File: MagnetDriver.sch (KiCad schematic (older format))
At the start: 54 parts, among them J1 MAGNET1, J2 MAGNET2, J3 INPUT_JACK, J4 PWR_IN, Q1 2N3904, Q2 TIP122, Q3 TIP32A, Q4 2N3904, Q5 TIP122, Q6 TIP32A, U1 LM324, U2 TEENSY_3.6_MINIMAL, U3 LM7805_TO220

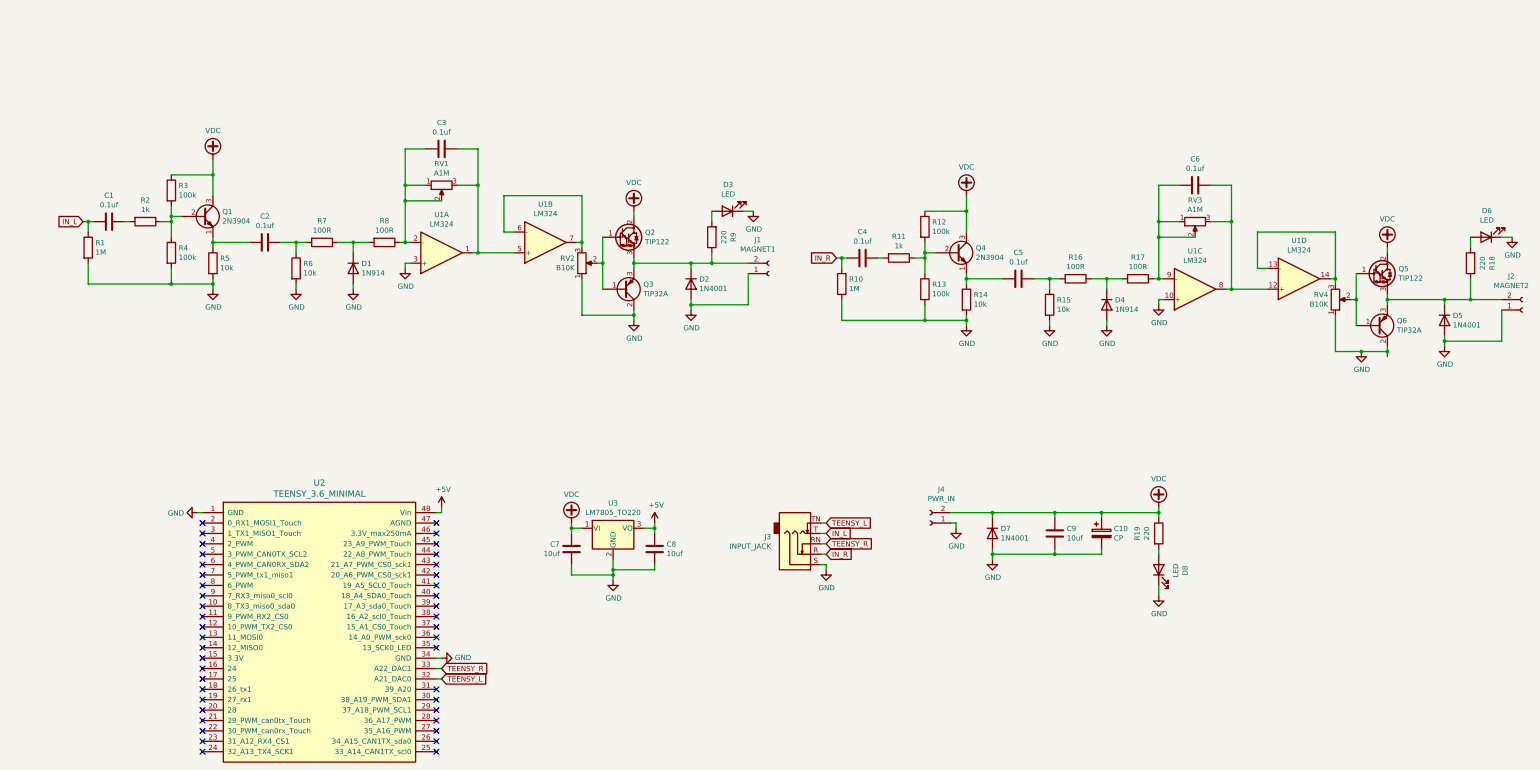
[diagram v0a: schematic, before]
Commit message: checked schematic + footprints
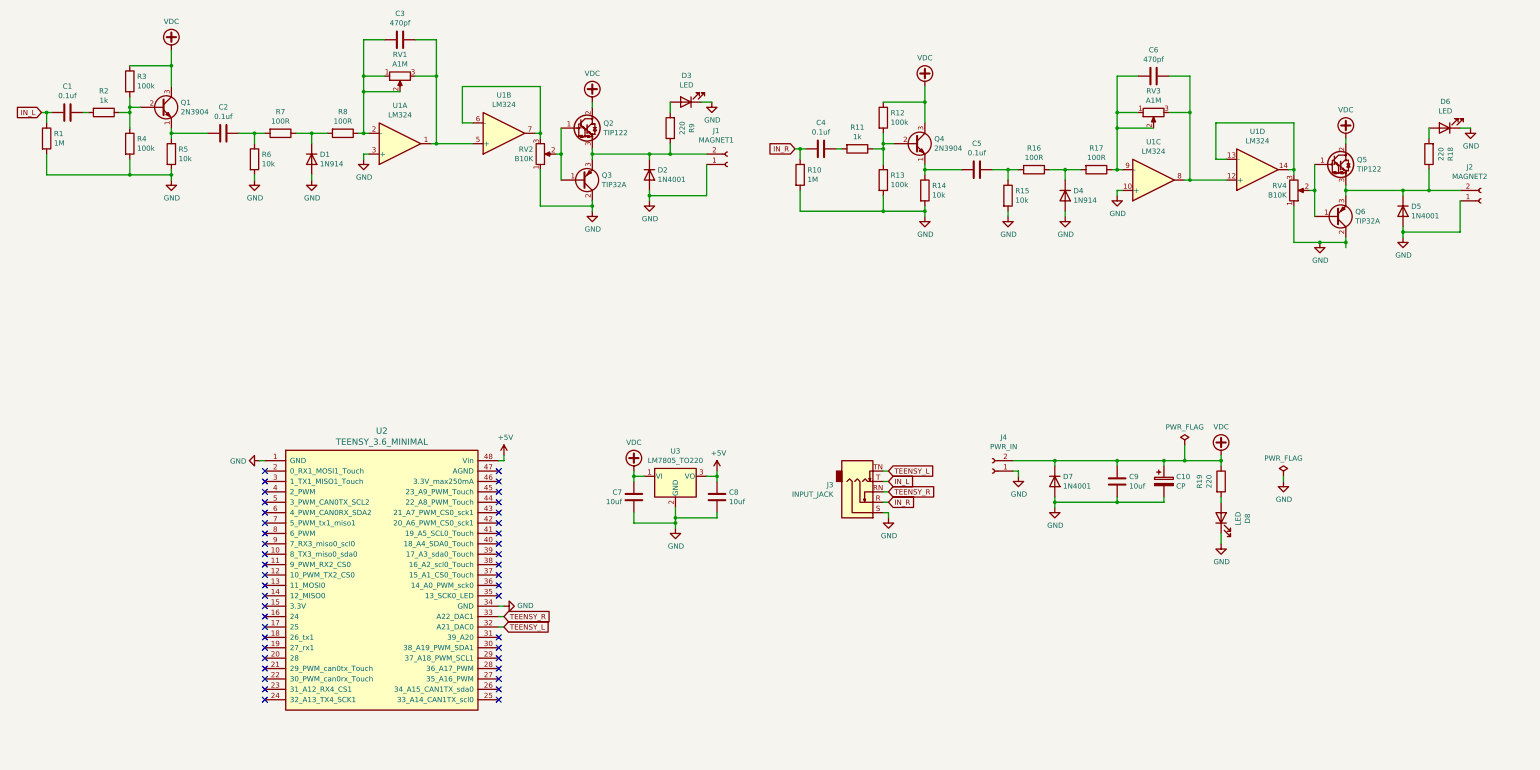
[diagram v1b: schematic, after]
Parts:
- C3, C6: value 0.1uf -> 470pf
- J3: footprint HammerheadAudio:Tayda_3.5mm_stereo_TRS_jack_A-853 -> HammerheadAudio:Tayda_SwitchedStereoJack-PJ-307
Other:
- moved on the sheet: C1, C10, C2, C3, C4, C5, C6, C7, C8, C9, D1, D2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
